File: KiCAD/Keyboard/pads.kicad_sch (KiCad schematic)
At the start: 18 parts

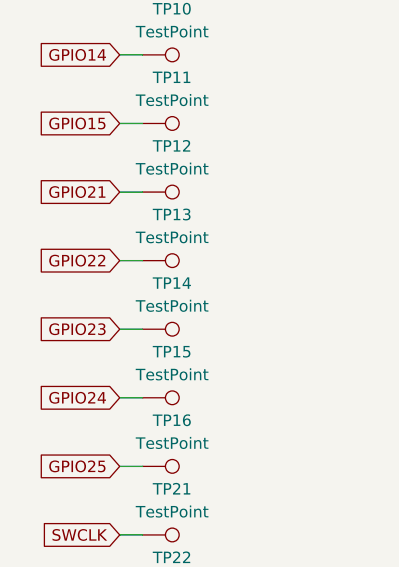
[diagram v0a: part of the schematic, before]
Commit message: idk what i did tbh
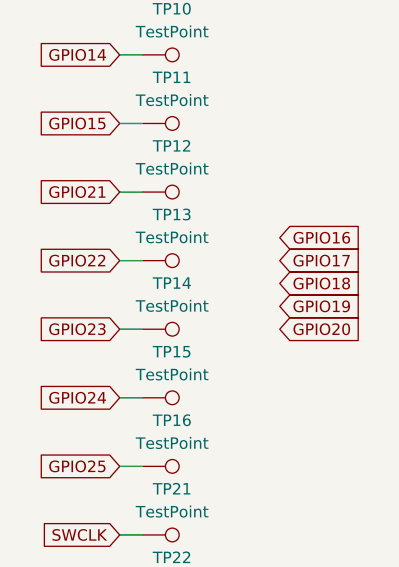
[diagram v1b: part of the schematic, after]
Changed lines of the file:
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@@
+		)
+	)
+	(global_label "GPIO18"
+		(shape input)
+		(at 54.61 123.19 0)
+		(fields_autoplaced yes)
+		(effects
+			(font
+				(size 1.27 1.27)
+			)
+			(justify left)
+		)
+		(property "Intersheetrefs" "${INTERSHEET_REFS}"
+			(at 64.4895 123.19 0)
+			(effects
+				(font
+					(size 1.27 1.27)
+				)
+				(justify left)
+				(hide yes)
+			)
 		)
 	)
@@
 		)
 	)
+	(global_label "GPIO20"
+		(shape input)
+		(at 54.61 128.27 0)
+		(fields_autoplaced yes)
+		(effects
+			(font
+				(size 1.27 1.27)
+			)
+			(justify left)
+		)
+		(property "Intersheetrefs" "${INTERSHEET_REFS}"
+			(at 64.4895 128.27 0)
+			(effects
+				(font
+					(size 1.27 1.27)
+				)
+				(justify left)
+				(hide yes)
+			)
+		)
+	)
+	(global_label "GPIO17"
+		(shape input)
+		(at 54.61 120.65 0)
+		(fields_autoplaced yes)
+		(effects
+			(font
+				(size 1.27 1.27)
+			)
+			(justify left)
+		)
+		(property "Intersheetrefs" "${INTERSHEET_REFS}"
+			(at 64.4895 120.65 0)
+			(effects
+				(font
+					(size 1.27 1.27)
+				)
+				(justify left)
+				(hide yes)
+			)
+		)
+	)
 	(global_label "GPIO10"
 		(shape input)
@@
 		)
 	)
+	(global_label "GPIO19"
+		(shape input)
+		(at 54.61 125.73 0)
+		(fields_autoplaced yes)
+		(effects
+			(font
+				(size 1.27 1.27)
+			)
+			(justify left)
+		)
+		(property "Intersheetrefs" "${INTERSHEET_REFS}"
+			(at 64.4895 125.73 0)
+			(effects
+				(font
+					(size 1.27 1.27)
+				)
+				(justify left)
+				(hide yes)
+			)
+		)
+	)
 	(global_label "GPIO23"
 		(shape input)
@@
 				(hide yes)
 			)
+		)
+	)
+	(global_label "GPIO16"
+		(shape input)
+		(at 54.61 118.11 0)
+		(fields_autoplaced yes)
+		(effects
+			(font
+				(size 1.27 1.27)
+			)
+			(justify left)
+		)
+		(property "Intersheetrefs" "${INTERSHEET_REFS}"
+			(at 64.4895 118.11 0)
+			(effects
+				(font
+					(size 1.27 1.27)
+				)
+				(justify left)
+				(hide yes)
+			)

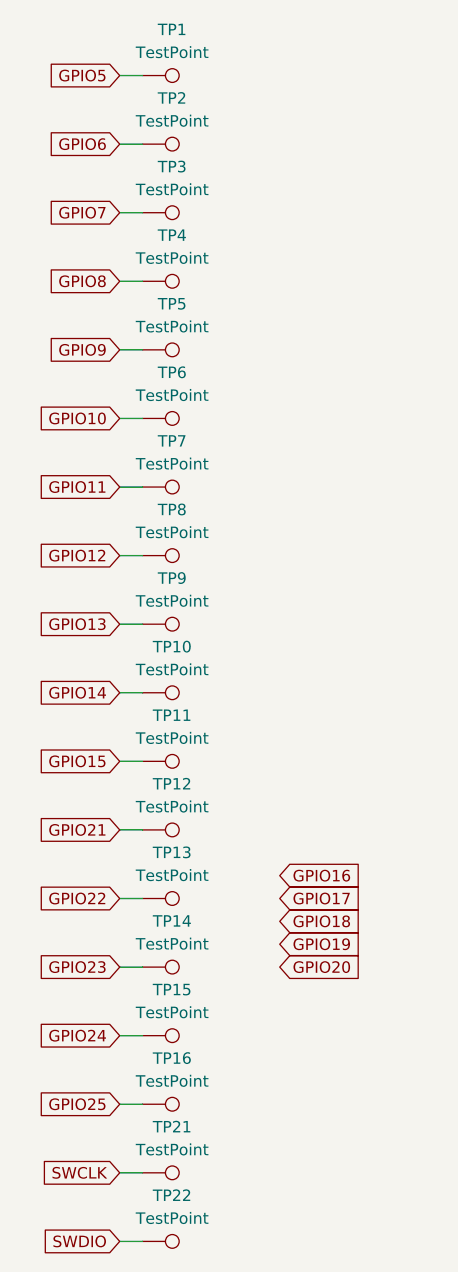
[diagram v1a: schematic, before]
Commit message: why no commit
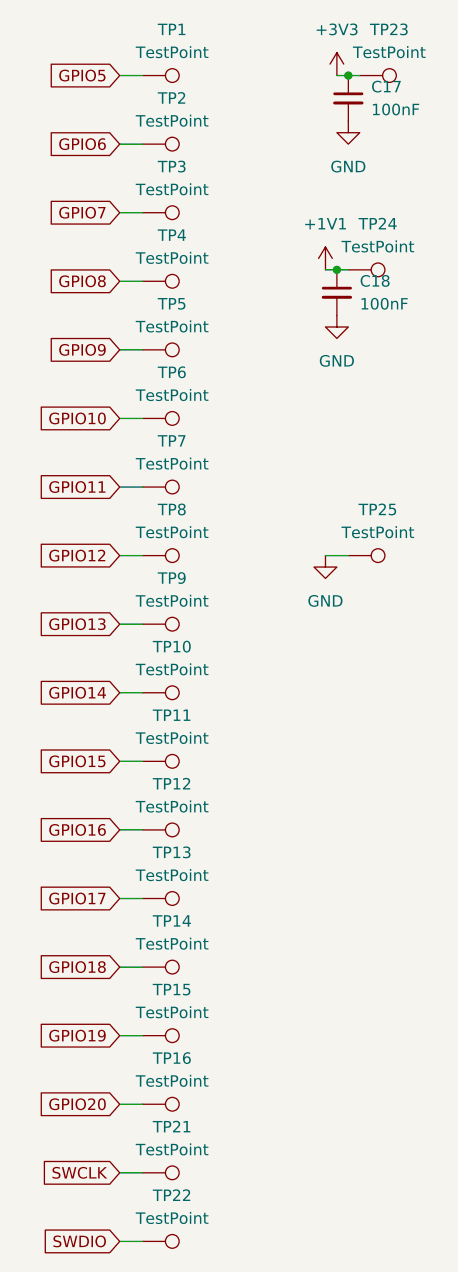
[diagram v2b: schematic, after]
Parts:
- added C17, C18: 100nF, Capacitor_SMD:C_0402_1005Metric, symbol Device:C_Small
- added TP23, TP24, TP25: TestPoint, TestPoint:TestPoint_Pad_D2.0mm, symbol Connector:TestPoint
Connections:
- net GPIO21 is gone; now on net GPIO16: TP12.1
- net GPIO22 is gone; now on net GPIO17: TP13.1
- net GPIO23 is gone; now on net GPIO18: TP14.1
- net GPIO24 is gone; now on net GPIO19: TP15.1
- net GPIO25 is gone; now on net GPIO20: TP16.1
- new net +1V1: C18.1, TP24.1
- new net +3V3: C17.1, TP23.1
- new net GND: C17.2, C18.2, TP25.1
